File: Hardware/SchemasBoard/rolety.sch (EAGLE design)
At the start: 29 parts, among them IC1 LNK302, IC3 MC33269ST-3.3T3, K1 FRS1B, K2 FRS1B, T1 BC846, T2 BC846

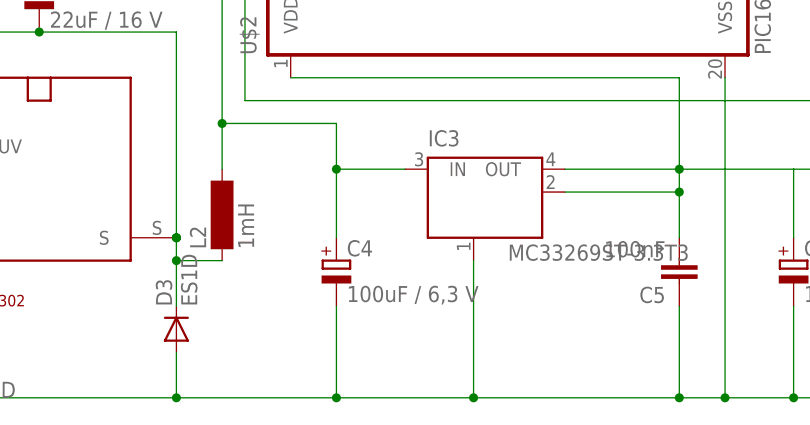
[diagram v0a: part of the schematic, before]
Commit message: aaa
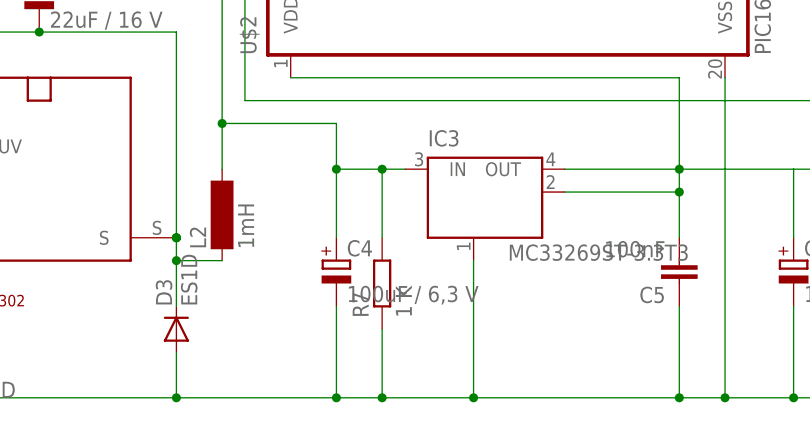
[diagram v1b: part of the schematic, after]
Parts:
- added R7: 1 K, resistor:R-EU_M2012
- C3: device resistor:CPOL-EUE2.5-5 -> resistor:CPOL-EUSMCC
- R2: device resistor:R-EU_R2512W -> resistor:R-EU_0411/12
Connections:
- net GND: now also R7.1
- net N$27: now also R7.2
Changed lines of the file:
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@@
 <grid distance="0.1" unitdist="inch" unit="inch" style="lines" multiple="1" display="no" altdistance="0.01" altunitdist="inch" altunit="inch"/>
 <layers>
-<layer number="1" name="Top" color="1" fill="1" visible="no" active="no"/>
-<layer number="16" name="Bottom" color="12" fill="1" visible="no" active="no"/>
-<layer number="17" name="Pads" color="2" fill="1" visible="no" active="no"/>
-<layer number="18" name="Vias" color="2" fill="1" visible="no" active="no"/>
-<layer number="19" name="Unrouted" color="6" fill="1" visible="no" active="no"/>
-<layer number="20" name="Dimension" color="15" fill="1" visible="no" active="no"/>
-<layer number="21" name="tPlace" color="15" fill="1" visible="no" active="no"/>
-<layer number="22" name="bPlace" color="11" fill="1" visible="no" active="no"/>
-<layer number="23" name="tOrigins" color="15" fill="1" visible="no" active="no"/>
-<layer number="24" name="bOrigins" color="15" fill="1" visible="no" active="no"/>
-<layer number="25" name="tNames" color="7" fill="1" visible="no" active="no"/>
-<layer number="26" name="bNames" color="7" fill="1" visible="no" active="no"/>
-<layer number="27" name="tValues" color="7" fill="1" visible="no" active="no"/>
-<layer number="28" name="bValues" color="7" fill="1" visible="no" active="no"/>
+<layer number="1" name="Top" color="1" fill="1" visible="yes" active="no"/>
+<layer number="16" name="Bottom" color="12" fill="1" visible="yes" active="no"/>
+<layer number="17" name="Pads" color="2" fill="1" visible="yes" active="no"/>
+<layer number="18" name="Vias" color="2" fill="1" visible="yes" active="no"/>
+<layer number="19" name="Unrouted" color="6" fill="1" visible="yes" active="no"/>
+<layer number="20" name="Dimension" color="15" fill="1" visible="yes" active="no"/>
+<layer number="21" name="tPlace" color="15" fill="1" visible="yes" active="no"/>
+<layer number="22" name="bPlace" color="11" fill="1" visible="yes" active="no"/>
+<layer number="23" name="tOrigins" color="15" fill="1" visible="yes" active="no"/>
+<layer number="24" name="bOrigins" color="15" fill="1" visible="yes" active="no"/>
+<layer number="25" name="tNames" color="7" fill="1" visible="yes" active="no"/>
+<layer number="26" name="bNames" color="7" fill="1" visible="yes" active="no"/>
+<layer number="27" name="tValues" color="7" fill="1" visible="yes" active="no"/>
+<layer number="28" name="bValues" color="7" fill="1" visible="yes" active="no"/>
 <layer number="29" name="tStop" color="7" fill="3" visible="no" active="no"/>
 <layer number="30" name="bStop" color="7" fill="6" visible="no" active="no"/>
@@
 <layer number="35" name="tGlue" color="7" fill="4" visible="no" active="no"/>
 <layer number="36" name="bGlue" color="7" fill="5" visible="no" active="no"/>
-<layer number="37" name="tTest" color="7" fill="1" visible="no" active="no"/>
-<layer number="38" name="bTest" color="7" fill="1" visible="no" active="no"/>
+<layer number="37" name="tTest" color="7" fill="1" visible="yes" active="no"/>
+<layer number="38" name="bTest" color="7" fill="1" visible="yes" active="no"/>
 <layer number="39" name="tKeepout" color="4" fill="11" visible="no" active="no"/>
 <layer number="40" name="bKeepout" color="1" fill="11" visible="no" active="no"/>
@@
 <layer number="44" name="Drills" color="7" fill="1" visible="no" active="no"/>
 <layer number="45" name="Holes" color="7" fill="1" visible="no" active="no"/>
-<layer number="46" name="Milling" color="3" fill="1" visible="no" active="no"/>
-<layer number="47" name="Measures" color="7" fill="1" visible="no" active="no"/>
-<layer number="48" name="Document" color="7" fill="1" visible="no" active="no"/>
-<layer number="49" name="Reference" color="7" fill="1" visible="no" active="no"/>
-<layer number="50" name="dxf" color="7" fill="1" visible="no" active="no"/>
-<layer number="51" name="tDocu" color="7" fill="1" visible="no" active="no"/>
-<layer number="52" name="bDocu" color="7" fill="1" visible="no" active="no"/>
+<layer number="46" name="Milling" color="3" fill="1" visible="yes" active="no"/>
+<layer number="47" name="Measures" color="7" fill="1" visible="yes" active="no"/>
+<layer number="48" name="Document" color="7" fill="1" visible="yes" active="no"/>
+<layer number="49" name="Reference" color="7" fill="1" visible="yes" active="no"/>
+<layer number="50" name="dxf" color="7" fill="1" visible="yes" active="no"/>
+<layer number="51" name="tDocu" color="7" fill="1" visible="yes" active="no"/>
+<layer number="52" name="bDocu" color="7" fill="1" visible="yes" active="no"/>
 <layer number="91" name="Nets" color="2" fill="1" visible="yes" active="yes"/>
 <layer number="92" name="Busses" color="1" fill="1" visible="yes" active="yes"/>
@@
 <part name="B1" library="rectifier" deviceset="RECTIFIER-" device="S40" value="RECTIFIER"/>
 <part name="R1" library="resistor" deviceset="R-EU_" device="R2512W" value="100"/>
-<part name="R2" library="resistor" deviceset="R-EU_" device="R2512W" value="8,2"/>
+<part name="R2" library="resistor" deviceset="R-EU_" device="0411/12" value="8,2"/>
 <part name="U$1" library="rfm70" deviceset="RFM70" device=""/>
 <part name="U$2" library="microchip" deviceset="PIC16F690*" device=""/>
@@
 <part name="R4" library="resistor" deviceset="R-EU_" device="M2012" value="2,05 k"/>
 <part name="R5" library="resistor" deviceset="R-EU_" device="M2012" value="1 K"/>
-<part name="C3" library="resistor" deviceset="CPOL-EU" device="E2.5-5" value="22uF / 16 V"/>
+<part name="C3" library="resistor" deviceset="CPOL-EU" device="SMCC" value="22uF / 16 V"/>
 <part name="C4" library="resistor" deviceset="CPOL-EU" device="E2.5-5" value="100uF / 6,3 V"/>
 <part name="C5" library="resistor" deviceset="C-EU" device="C2012" value="100nF"/>
@@
 <part name="IC3" library="linear" deviceset="MC33269ST*" device="" technology="-3.3T3"/>
 <part name="L2" library="inductor-neosid" deviceset="BS" device="11" value="1mH"/>
+<part name="R7" library="resistor" deviceset="R-EU_" device="M2012" value="1 K"/>
 </parts>
 <sheets>
@@
 <instance part="IC3" gate="G$1" x="104.14" y="50.8"/>
 <instance part="L2" gate="G$1" x="76.2" y="50.8" rot="R90"/>
+<instance part="R7" gate="G$1" x="93.98" y="43.18" rot="R90"/>
 </instances>
 <busses>
@@
 <wire x1="22.86" y1="30.48" x2="71.12" y2="30.48" width="0.1524" layer="91"/>
 <wire x1="71.12" y1="30.48" x2="88.9" y2="30.48" width="0.1524" layer="91"/>
-<wire x1="88.9" y1="30.48" x2="104.14" y2="30.48" width="0.1524" layer="91"/>
+<wire x1="88.9" y1="30.48" x2="93.98" y2="30.48" width="0.1524" layer="91"/>
+<wire x1="93.98" y1="30.48" x2="104.14" y2="30.48" width="0.1524" layer="91"/>
 <wire x1="104.14" y1="30.48" x2="127" y2="30.48" width="0.1524" layer="91"/>
 <wire x1="127" y1="30.48" x2="132.08" y2="30.48" width="0.1524" layer="91"/>
@@
 <wire x1="104.14" y1="45.72" x2="104.14" y2="30.48" width="0.1524" layer="91"/>
 <junction x="104.14" y="30.48"/>
+<pinref part="R7" gate="G$1" pin="1"/>
+<wire x1="93.98" y1="38.1" x2="93.98" y2="30.48" width="0.1524" layer="91"/>
+<junction x="93.98" y="30.48"/>
 </segment>
 </net>
@@
 <wire x1="33.02" y1="83.82" x2="76.2" y2="83.82" width="0.1524" layer="91"/>
 <wire x1="0" y1="81.28" x2="0" y2="83.82" width="0.1524" layer="91"/>
-<wire x1="96.52" y1="55.88" x2="88.9" y2="55.88" width="0.1524" layer="91"/>
+<wire x1="96.52" y1="55.88" x2="93.98" y2="55.88" width="0.1524" layer="91"/>
+<wire x1="93.98" y1="55.88" x2="88.9" y2="55.88" width="0.1524" layer="91"/>
 <wire x1="76.2" y1="60.96" x2="88.9" y2="60.96" width="0.1524" layer="91"/>
 <wire x1="88.9" y1="60.96" x2="88.9" y2="55.88" width="0.1524" layer="91"/>
@@
 <wire x1="76.2" y1="55.88" x2="76.2" y2="60.96" width="0.1524" layer="91"/>
 <junction x="76.2" y="60.96"/>
-</segment>
-</net>
+<pinref part="R7" gate="G$1" pin="2"/>
+<wire x1="93.98" y1="48.26" x2="93.98" y2="55.88" width="0.1524" layer="91"/>
+<junction x="93.98" y="55.88"/>
+</segment>
+</net>
